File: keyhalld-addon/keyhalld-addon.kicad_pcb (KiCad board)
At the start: 4 copper layers, 120 x 39.5 mm, 48 parts, among them J1 Conn_01x06_Pin, J2 USB_C_Receptacle_USB2.0_16P, J3 Conn_01x04_Pin, SW1 SW_Push, SW2 SW_Push, SW3 SW_Push, SW4 SW_Push, SW5 SW_Push, SW6 SW_Push, SW7 SW_Push, SW8 SW_Push, U1 TLV1117-33, U2 RP2350A, U3 USBLC6-2SC6, U4 ER_OLEDM0.91_1x-I2C, Y1 12MHz

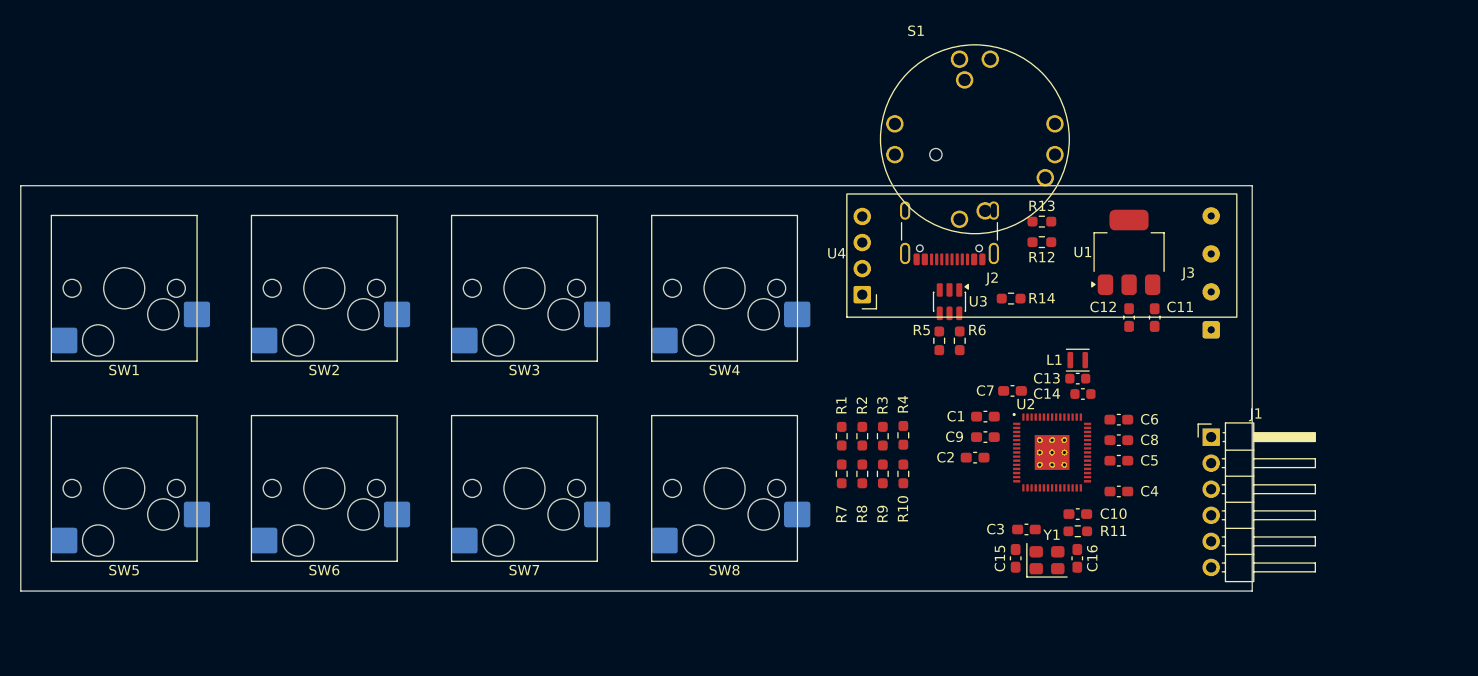
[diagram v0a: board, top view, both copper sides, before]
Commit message: maybe last schematic changes; pcb new layout
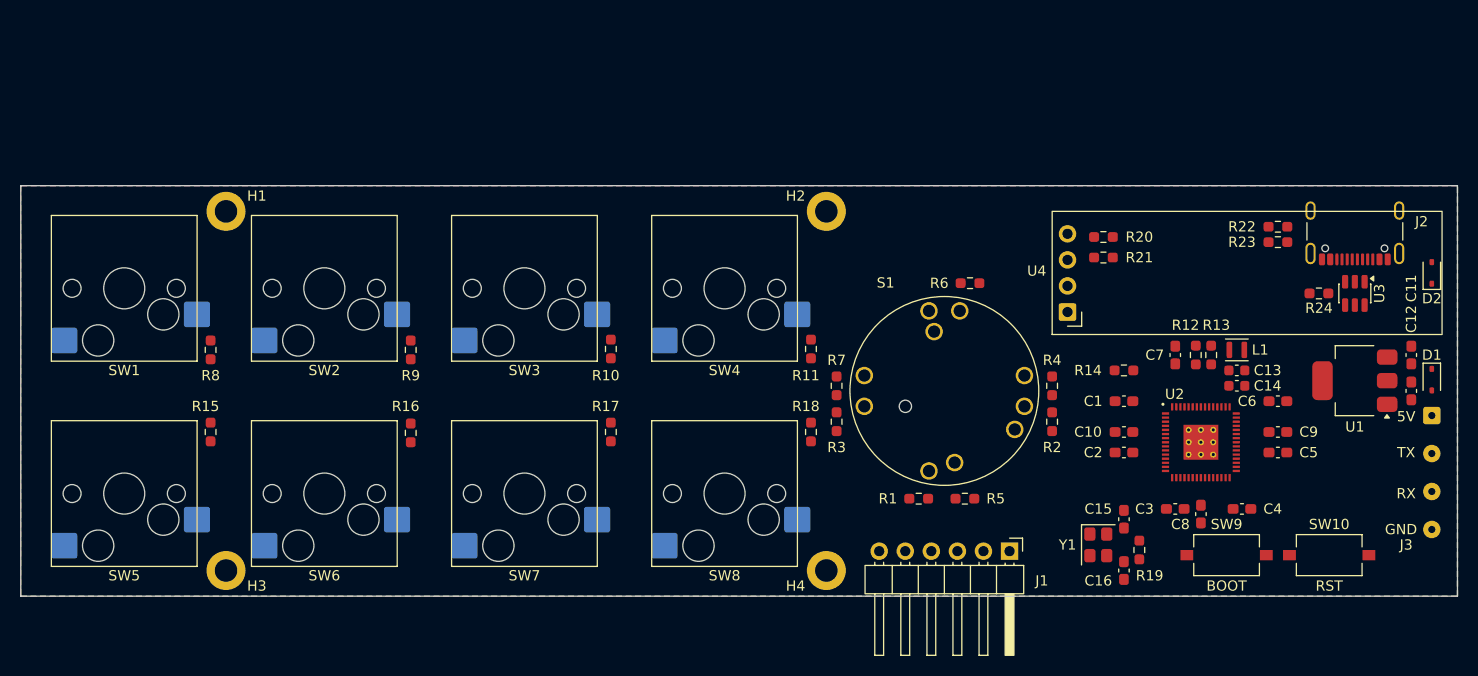
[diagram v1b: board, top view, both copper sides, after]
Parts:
- added D1: D, Diode_SMD:D_SOD-323, F.Cu at (187.5, 98.9)
- added D2: D, Diode_SMD:D_SOD-323, F.Cu at (187.5, 88.5)
- added H1: MountingHole_Pad, MountingHole:MountingHole_2.2mm_M2_DIN965_Pad, F.Cu at (70.0, 82.5)
- added H2: MountingHole_Pad, MountingHole:MountingHole_2.2mm_M2_DIN965_Pad, F.Cu at (128.5, 82.5)
- added H3: MountingHole_Pad, MountingHole:MountingHole_2.2mm_M2_DIN965_Pad, F.Cu at (70.0, 117.5)
- added H4: MountingHole_Pad, MountingHole:MountingHole_2.2mm_M2_DIN965_Pad, F.Cu at (128.5, 117.5)
- added R15: 10K, Resistor_SMD:R_0603_1608Metric_Pad0.98x0.95mm_HandSolder, F.Cu at (68.5, 104.0)
- added R16: 10K, Resistor_SMD:R_0603_1608Metric_Pad0.98x0.95mm_HandSolder, F.Cu at (88.0, 104.1)
- added R17: 10K, Resistor_SMD:R_0603_1608Metric_Pad0.98x0.95mm_HandSolder, F.Cu at (107.5, 104.0)
- added R18: 10K, Resistor_SMD:R_0603_1608Metric_Pad0.98x0.95mm_HandSolder, F.Cu at (127.0, 104.0)
- added R19: 1K, Resistor_SMD:R_0603_1608Metric_Pad0.98x0.95mm_HandSolder, F.Cu at (159.0, 115.5)
- added R20: 4K7, Resistor_SMD:R_0603_1608Metric_Pad0.98x0.95mm_HandSolder, F.Cu at (155.5, 85.0)
- added R21: 4K7, Resistor_SMD:R_0603_1608Metric_Pad0.98x0.95mm_HandSolder, F.Cu at (155.5, 87.0)
- added R22: 5K1, Resistor_SMD:R_0603_1608Metric_Pad0.98x0.95mm_HandSolder, F.Cu at (172.5, 84.0)
- added R23: 5K1, Resistor_SMD:R_0603_1608Metric_Pad0.98x0.95mm_HandSolder, F.Cu at (172.5, 85.5)
- added R24: 1.5K, Resistor_SMD:R_0603_1608Metric_Pad0.98x0.95mm_HandSolder, F.Cu at (176.5, 90.5)
- added SW10: RST, Button_Switch_SMD:SW_Tactile_SPST_NO_Straight_CK_PTS636Sx25SMTRLFS, F.Cu at (177.5, 116.0)
- added SW9: BOOT, Button_Switch_SMD:SW_Tactile_SPST_NO_Straight_CK_PTS636Sx25SMTRLFS, F.Cu at (167.5, 116.0)
- R11: value 1K -> 10K
- R12, R13: value 5K1 -> 22R
- R14: value 1.5K -> 4K7
- R5, R6: value 22R -> 10K
- moved R8 64.6 mm to (68.5, 96.0), turned to 90 degrees
- moved R9 47.6 mm to (88.0, 96.0), turned to 90 degrees
- moved U3 39.5 mm to (180.0, 90.5)
- moved J2 39.5 mm to (180.0, 83.5)
- moved R11 31.5 mm to (127.0, 95.9), turned to 90 degrees
- moved R10 31.0 mm to (107.5, 95.9), turned to 90 degrees
- moved C9 28.5 mm to (172.5, 104.0), turned to 0 degrees
- moved C12 28.4 mm to (185.5, 100.0)
- moved U1 25.3 mm to (180.0, 99.0), turned to 180 degrees
- moved C11 25.3 mm to (185.5, 96.5), turned to 90 degrees
- moved S1 24.7 mm to (140.0, 100.0)
- moved J3 23.1 mm to (187.5, 102.4), turned to -90 degrees
- moved J1 22.6 mm to (146.3, 115.6), turned to -90 degrees
- moved R13 21.0 mm to (166.0, 96.5), turned to -90 degrees
- moved U4 20.1 mm to (152.0, 92.3)
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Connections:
- J2 pad A4: +5V -> Net-(D2-A)
- J2 pad A9: +5V -> Net-(D2-A)
- J2 pad B4: +5V -> Net-(D2-A)
- J2 pad B9: +5V -> Net-(D2-A)
- J3 pad 1: +5V -> Net-(D1-K)
- R1 pad 2: KEY1 -> EN_S_A
- R10 pad 2: KEY8 -> KEY3
- R11 pad 1: XOUT -> +3.3V
- R11 pad 2: Net-(C16-Pad2) -> KEY4
- R12 pad 1: Net-(J2-CC1) -> Net-(U2-USB_DP)
- R12 pad 2: GND -> D+
- R13 pad 1: GND -> D-
- R13 pad 2: Net-(J2-CC2) -> Net-(U2-USB_DM)
- R14 pad 1: /CONN_D+ -> Net-(U2-QSPI_~{SS})
- R14 pad 2: +3.3V -> BOOT
- R2 pad 1: +3.3V -> EN_S_B
- R2 pad 2: KEY2 -> +3.3V
- R3 pad 2: KEY3 -> EN_A
- R4 pad 1: +3.3V -> EN_B
- R4 pad 2: KEY4 -> +3.3V
- R5 pad 1: Net-(U2-USB_DP) -> +3.3V
- R5 pad 2: D+ -> EN_S_P
- R6 pad 1: D- -> EN_S_C
- R6 pad 2: Net-(U2-USB_DM) -> +3.3V
- R7 pad 2: KEY5 -> EN_S_D
- R8 pad 2: KEY6 -> KEY1
- R9 pad 2: KEY7 -> KEY2
- S1 pad A: unconnected-(S1-PadA) -> EN_S_A
- S1 pad B: unconnected-(S1-PadB) -> EN_S_B
- S1 pad C: unconnected-(S1-PadC) -> EN_S_C
- S1 pad COM: unconnected-(S1-PadCOM) -> GND
- S1 pad D: unconnected-(S1-PadD) -> EN_S_D
- S1 pad EN_A: unconnected-(S1-PadEN_A) -> EN_A
- S1 pad EN_B: unconnected-(S1-PadEN_B) -> EN_B
- S1 pad EN_COM: unconnected-(S1-PadEN_COM) -> GND
- S1 pad GND: unconnected-(S1-PadGND) -> GND
- S1 pad P: unconnected-(S1A-PUSH-PadP) -> EN_S_P
- U2 pad 31: unconnected-(U2-GPIO19-Pad31) -> EN_A
- U2 pad 32: unconnected-(U2-GPIO20-Pad32) -> EN_B
- U2 pad 33: unconnected-(U2-GPIO21-Pad33) -> EN_S_P
- U2 pad 34: unconnected-(U2-GPIO22-Pad34) -> EN_S_A
- U2 pad 35: unconnected-(U2-GPIO23-Pad35) -> EN_S_B
- U2 pad 36: unconnected-(U2-GPIO24-Pad36) -> EN_S_C
- U2 pad 37: unconnected-(U2-GPIO25-Pad37) -> EN_S_D
- U2 pad 59: unconnected-(U2-QSPI_SD1-Pad59) -> GND
- U2 pad 60: unconnected-(U2-QSPI_~{SS}-Pad60) -> Net-(U2-QSPI_~{SS})
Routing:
- added copper zone on B.Cu, net GND
- added copper zone on F.Cu, net GND
- added copper zone on In1.Cu, net GND
- added copper zone on In2.Cu, net GND
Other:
- board size 120 x 39.5 mm -> 140 x 40 mm
- board text added: "5V"
- board text added: "GND"
- board text added: "RX"
- board text added: "TX"
